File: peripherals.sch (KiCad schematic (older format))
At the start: 36 parts, among them J10 CT0, J4 IDE, J7 PIO Header, J8 Port A, J9 Port A, U7 Z84C2010AEG, U8 Z84C4310AEG, U9 Z84C3010AEG

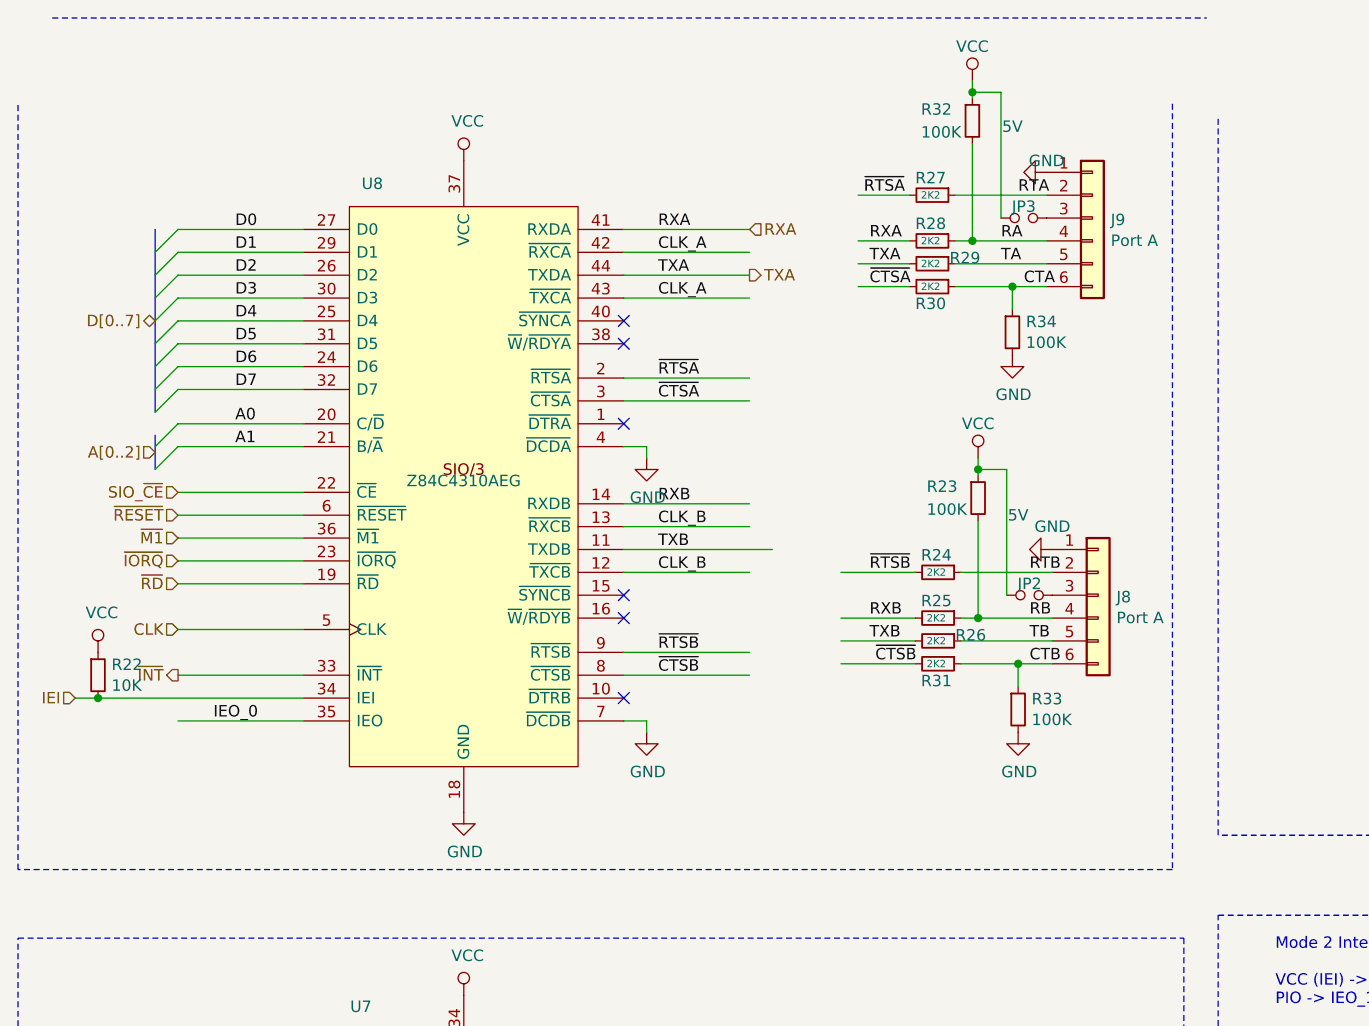
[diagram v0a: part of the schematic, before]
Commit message: lots of fixes
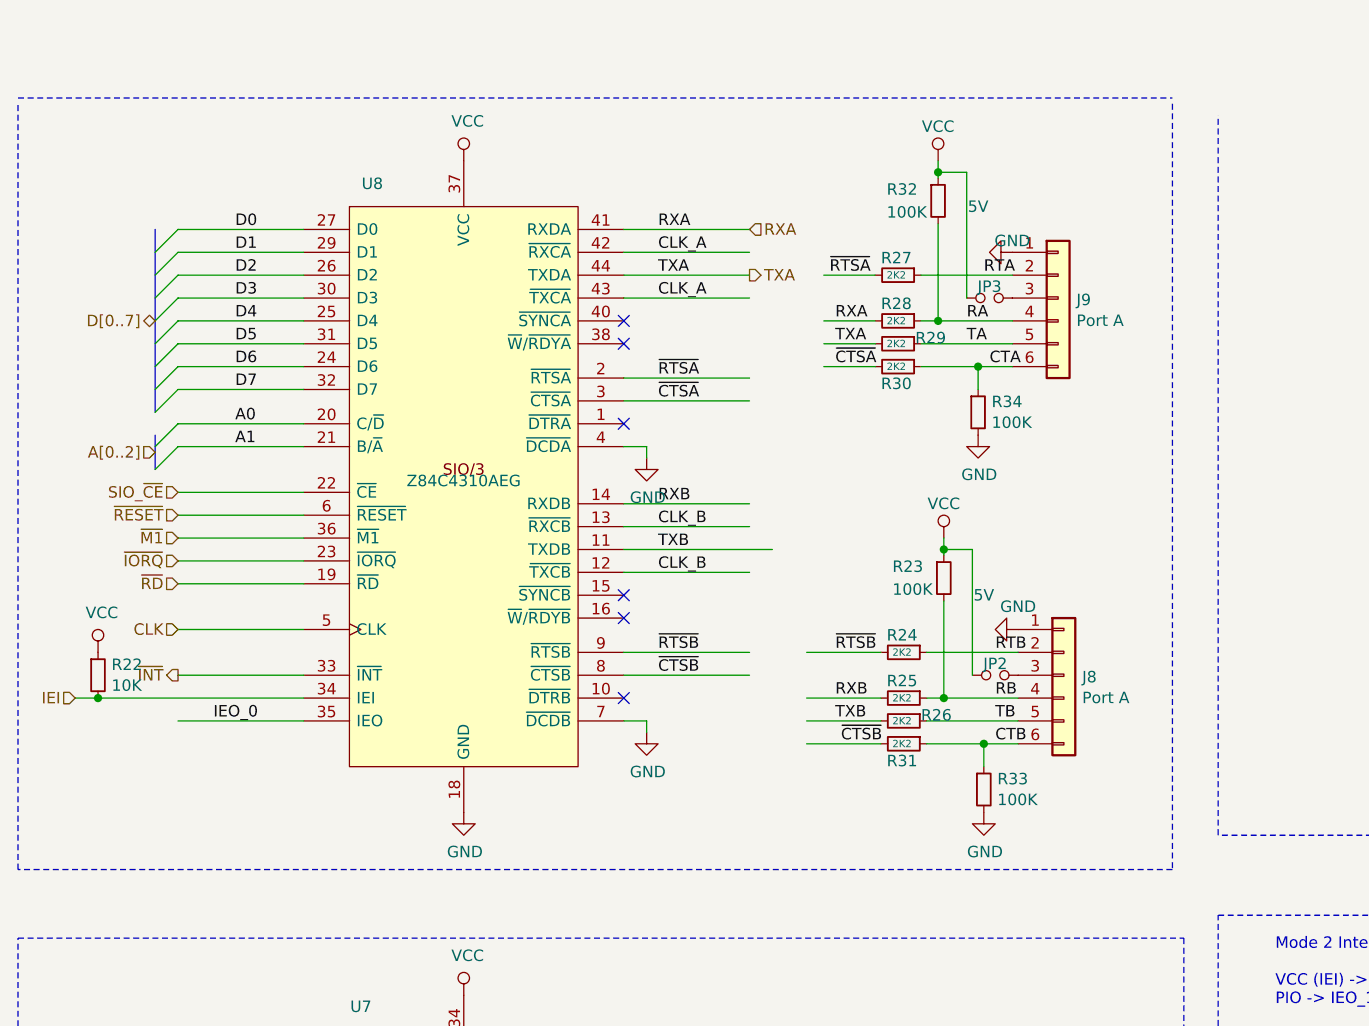
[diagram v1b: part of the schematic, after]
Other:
- moved on the sheet: J8, J9, JP2, JP3, R23, R24, R25, R26, R27, R28, R29, R30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
